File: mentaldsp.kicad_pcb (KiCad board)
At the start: 2 copper layers, 125 x 35 mm, 30 parts, among them J5 NEMA Conn, J7 NEMA Conn, J8 NEMA Conn, J9 Barrel_Jack_Switch, U6 ESP32-S3-SUPERMINI, U7 TMC2209_N0, U8 TMC2209_N2, U9 TMC2209_N1

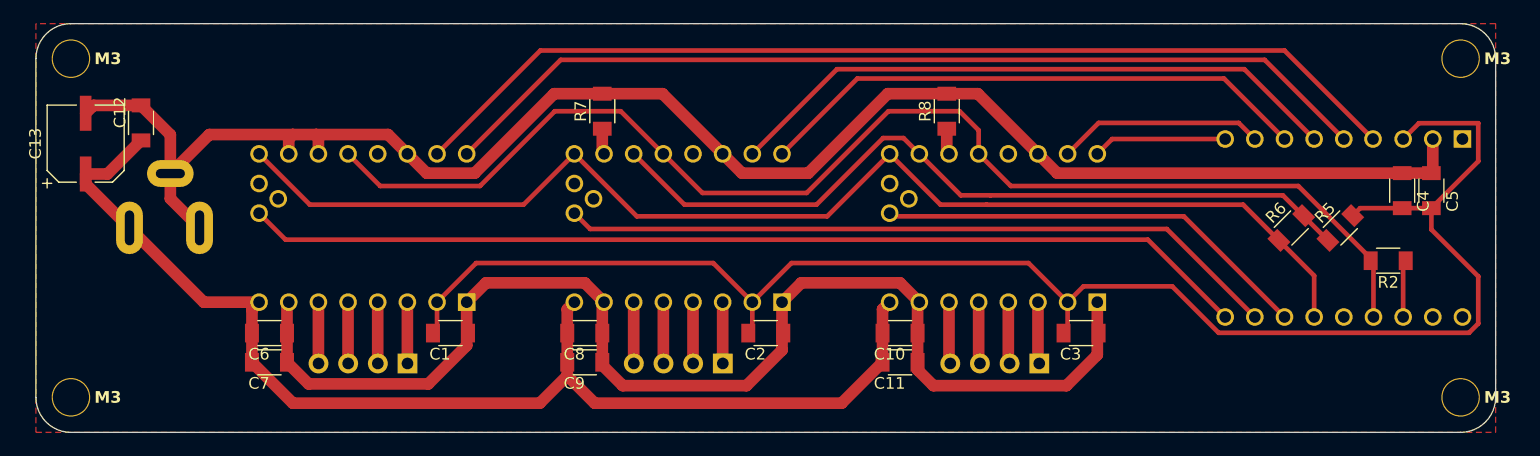
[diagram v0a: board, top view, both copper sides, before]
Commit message: gerber
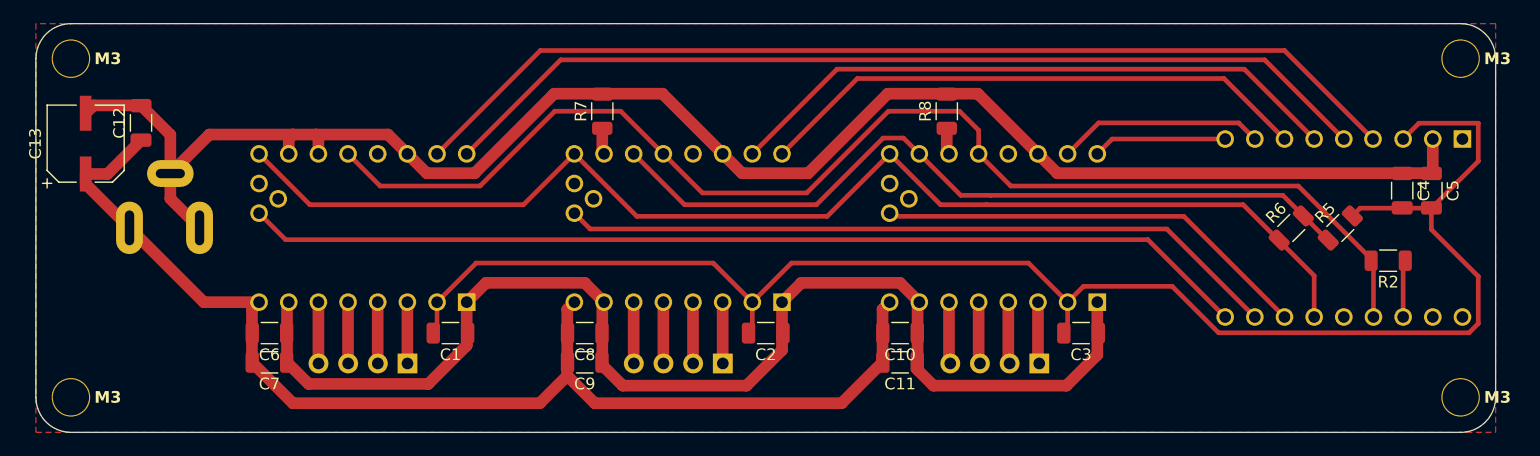
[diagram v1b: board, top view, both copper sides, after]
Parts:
- C1, C10, C11, C12, C2, C3, C4, C5, C6, C7, C8, C9: footprint PCM_fab:C_1206 -> Capacitor_SMD:C_1206_3216Metric
- R2, R5, R6, R7, R8: footprint PCM_fab:R_1206 -> Resistor_SMD:R_1206_3216Metric
